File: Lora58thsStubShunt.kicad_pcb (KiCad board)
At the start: 2 copper layers, 35.5 x 18.5 mm, 9 parts, among them J1 Conn_Coaxial, J2 Conn_01x01_Pin, J3 Conn_01x01_Pin, J4 Conn_01x01_Pin

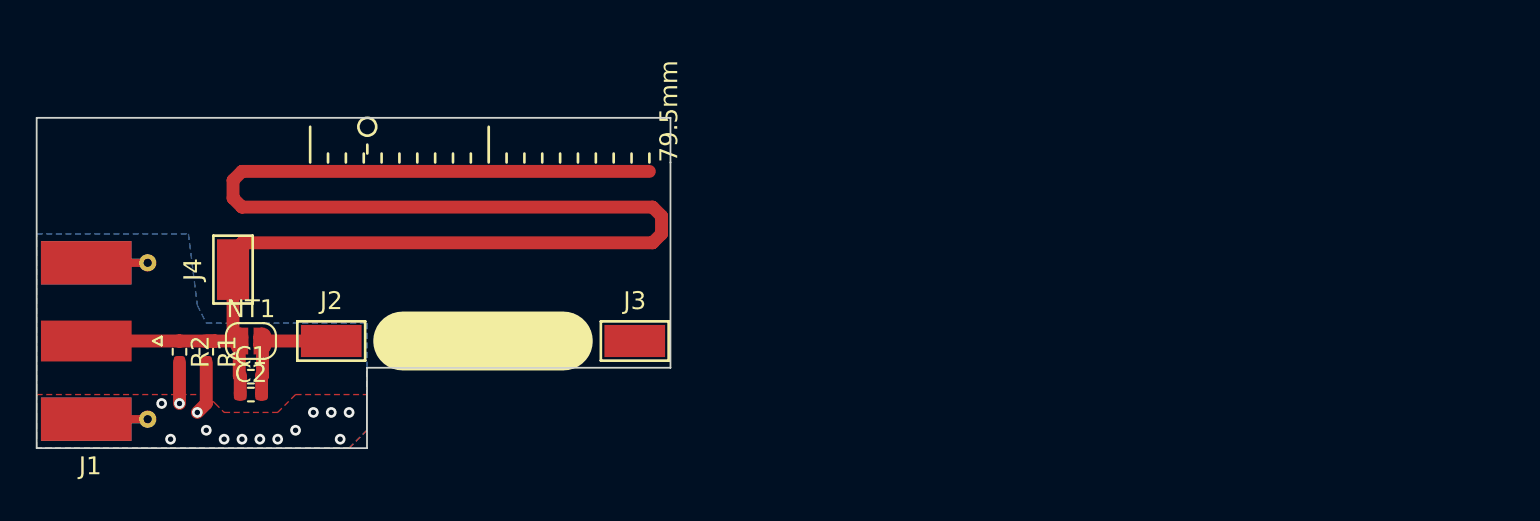
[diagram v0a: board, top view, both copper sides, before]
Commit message: Release Candidate
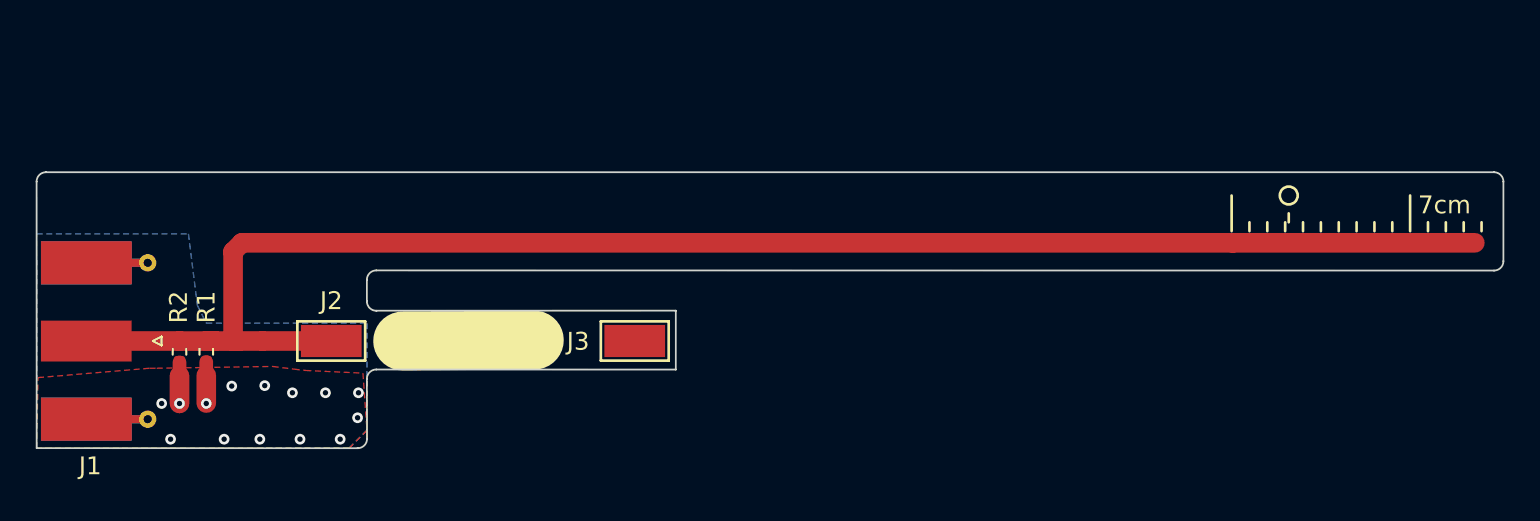
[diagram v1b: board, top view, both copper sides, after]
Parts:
- removed C1, C2: C_Small, Resistor_SMD:R_0402_1005Metric_Pad0.72x0.64mm_HandSolder
- removed J4: Conn_01x01_Pin, TestPoint:TestPoint_Keystone_5015_Micro-Minature
- removed NT1: NetTie_2, Jumper:SolderJumper-2_P1.3mm_Open_RoundedPad1.0x1.5mm
- R1: value R60 -> 60R
- R2: value R5 -> 5R
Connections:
- J2 pad 1: Net-(J2-Pin_1) -> Net-(J1-In)
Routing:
- net Net-(J2-Pin_1): track 6.87 -> 0.00 mm
- net Net-(J1-In): track 91.6 -> 89.0 mm
- net GND: track 5.31 -> 4.60 mm
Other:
- board size 35.5 x 18.5 mm -> 82.2 x 15.5 mm
- board text added: "7cm"
- board text added: "Trace thickness designed for 0.6mm board"
- board text removed: "79.5mm"
